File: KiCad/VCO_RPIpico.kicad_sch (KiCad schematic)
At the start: 92 parts, among them J1 AudioJack, J2 Power Jack, SW1 LFO1/2, SW2 Select LFO WaveForm, SW3 Fire4, SW4 Fire3, SW5 Fire2, SW6 Fire1, SW7 Shift2/Save, SW8 Shift1 / Select Bank, U2 PT2399, U3 L7805, sw10 sw_led_fire2, sw11 sw_led_fire3, sw12 sw_led_fire4, sw9 sw_led_fire1

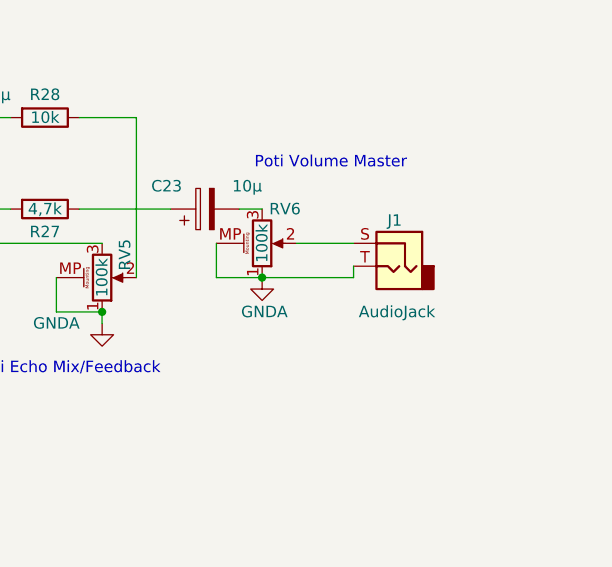
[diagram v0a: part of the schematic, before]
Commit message: CAD und eCAD
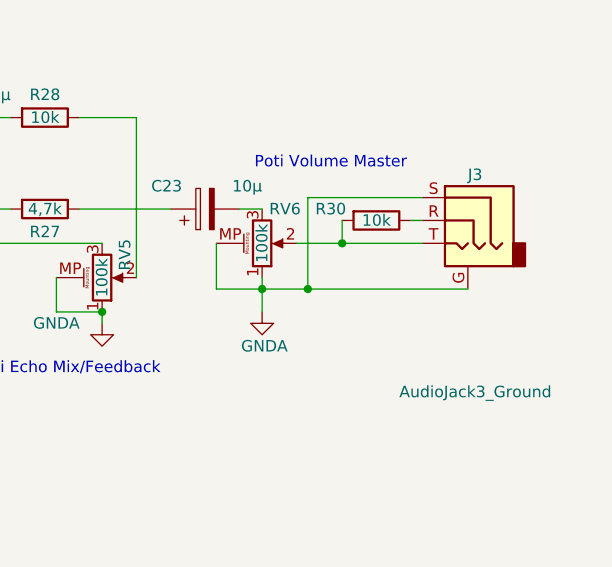
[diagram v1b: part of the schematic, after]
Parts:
- removed J1: AudioJack, Connector_Audio:Jack_3.5mm_Ledino_KB3SPRS_Horizontal, symbol Connector:AudioJack2
- added J3: AudioJack3_Ground, symbol Connector_Audio:AudioJack3_Ground
- added R30: 10k, Resistor_SMD:R_1206_3216Metric, symbol Device:R
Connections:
- net GND: now also J3.G, J3.S
- net at RV6.2: now also J3.T, R30.2
- new net: J3.R, R30.1
